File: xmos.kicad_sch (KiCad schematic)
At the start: 64 parts, among them Q1 LBSS138WT1G, Q2 BC847B, U10 SN74LVC125APWR, U7 XU316-1024-QF60B-C24, U8 W25Q128JVSIQ, U9 TLV73333PDBVR, Y2 24MHz

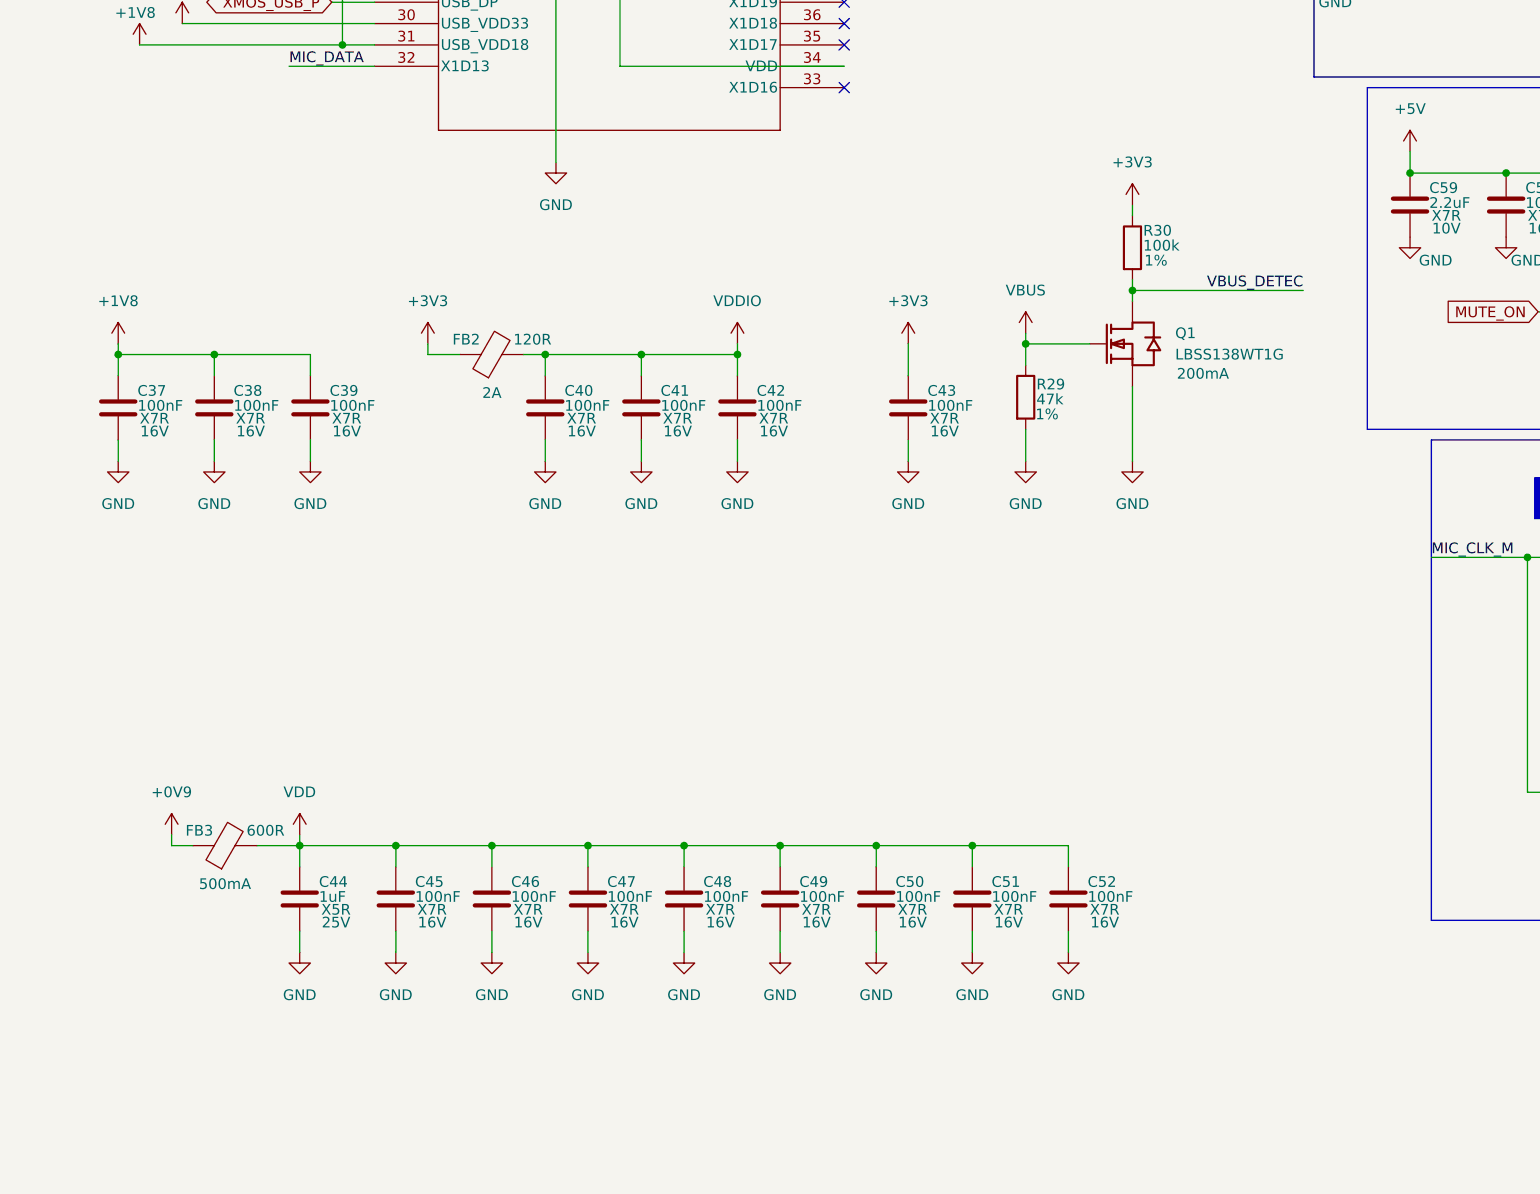
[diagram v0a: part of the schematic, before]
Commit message: rev2 update
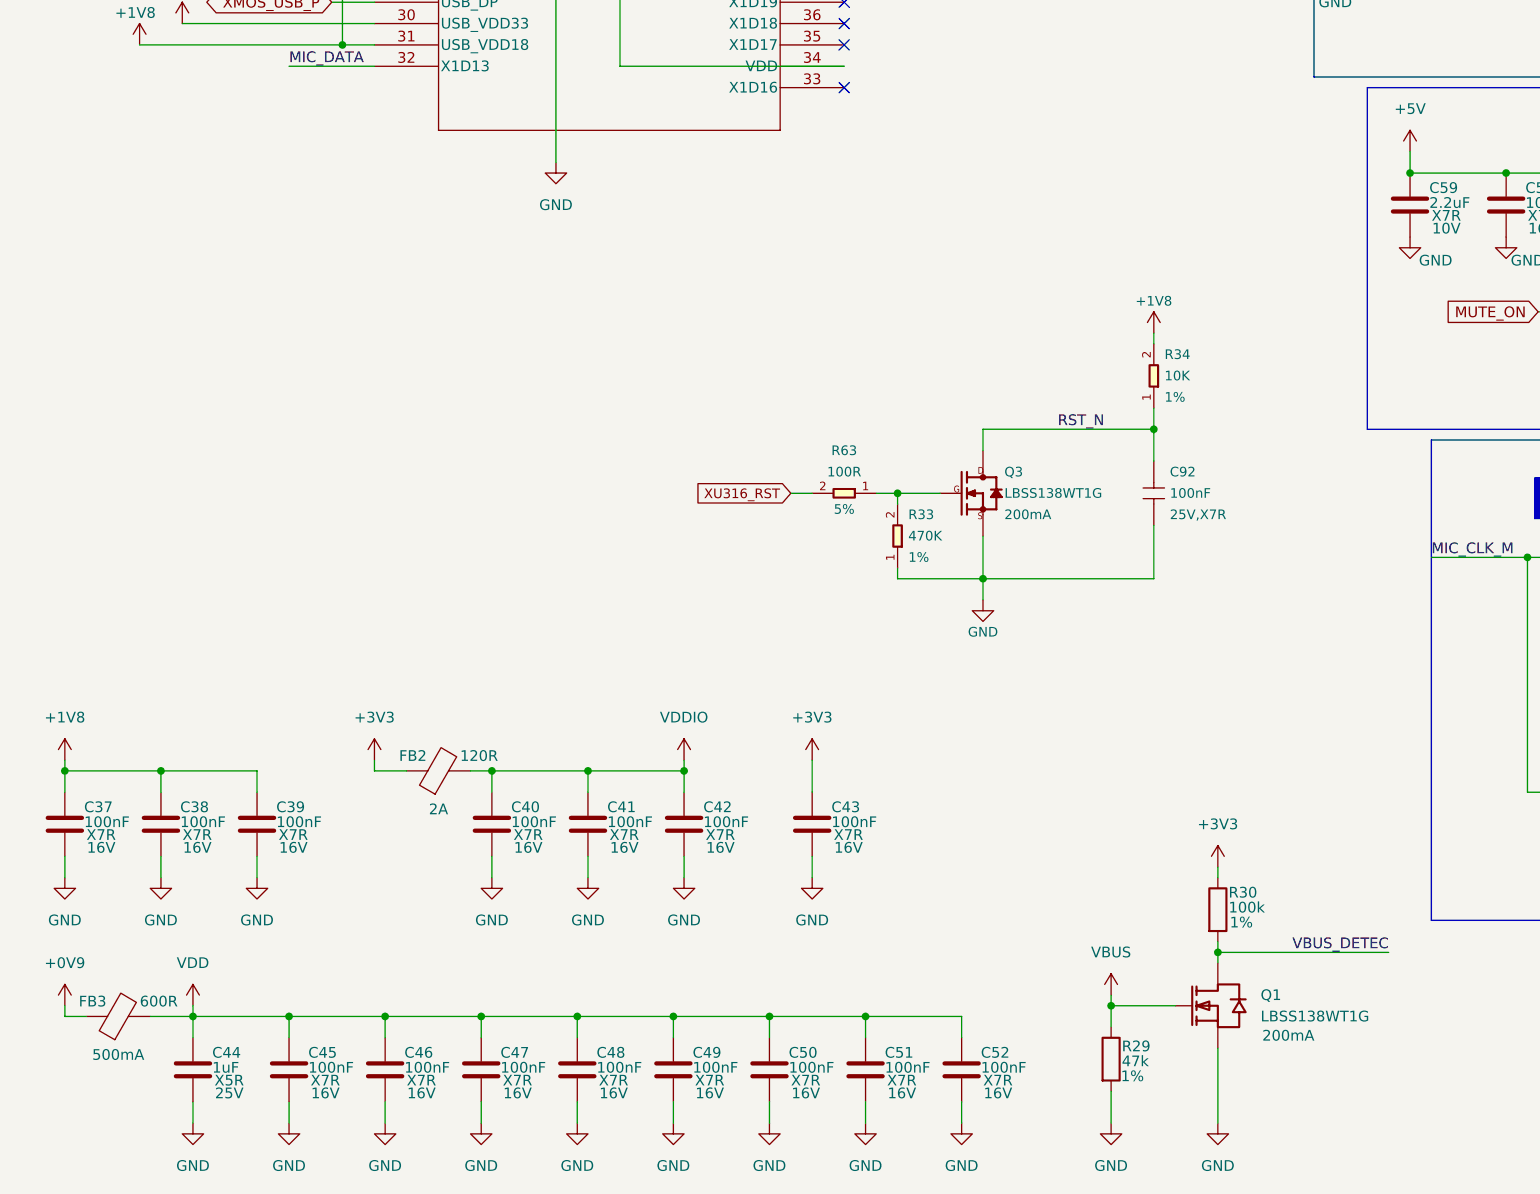
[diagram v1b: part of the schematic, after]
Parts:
- added C92: 100nF, Capacitor_SMD:C_0402_1005Metric, symbol Seeed_libadl:Capacitors/302010024
- added Q3: LBSS138WT1G, Package_TO_SOT_SMD:SOT-323_SC-70, symbol Seeed_libadl:Mosfet/305031542
- added R33: 470K, Resistor_SMD:R_0402_1005Metric, symbol Seeed_libdb:Resistors/301010069
- added R34: 10K, Resistor_SMD:R_0402_1005Metric, symbol Seeed_libadl:Resistors/301010047
- added R63: 100R, Resistor_SMD:R_0402_1005Metric, symbol Seeed_libadl:Resistors/301010028
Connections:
- net +1V8: now also R34.2
- net GND: now also C92.2, Q3.2 (S), R33.1
- net RST_N: now also C92.1, Q3.3 (D), R34.1
- new net: Q3.1 (G), R33.2, R63.1
- new net XU316_RST: R63.2
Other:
- moved on the sheet: C37, C38, C39, C40, C41, C42, C43, C44, C45, C46, C47, C48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
